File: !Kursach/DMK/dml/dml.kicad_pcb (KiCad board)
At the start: 2 copper layers, 64.7 x 68.8 mm, 26 parts, among them J1 Debug, J2 Conn_01x01_Male, J3 USB, SW1 SW_Push, SW2 SW_Push, U1 HEF4093B

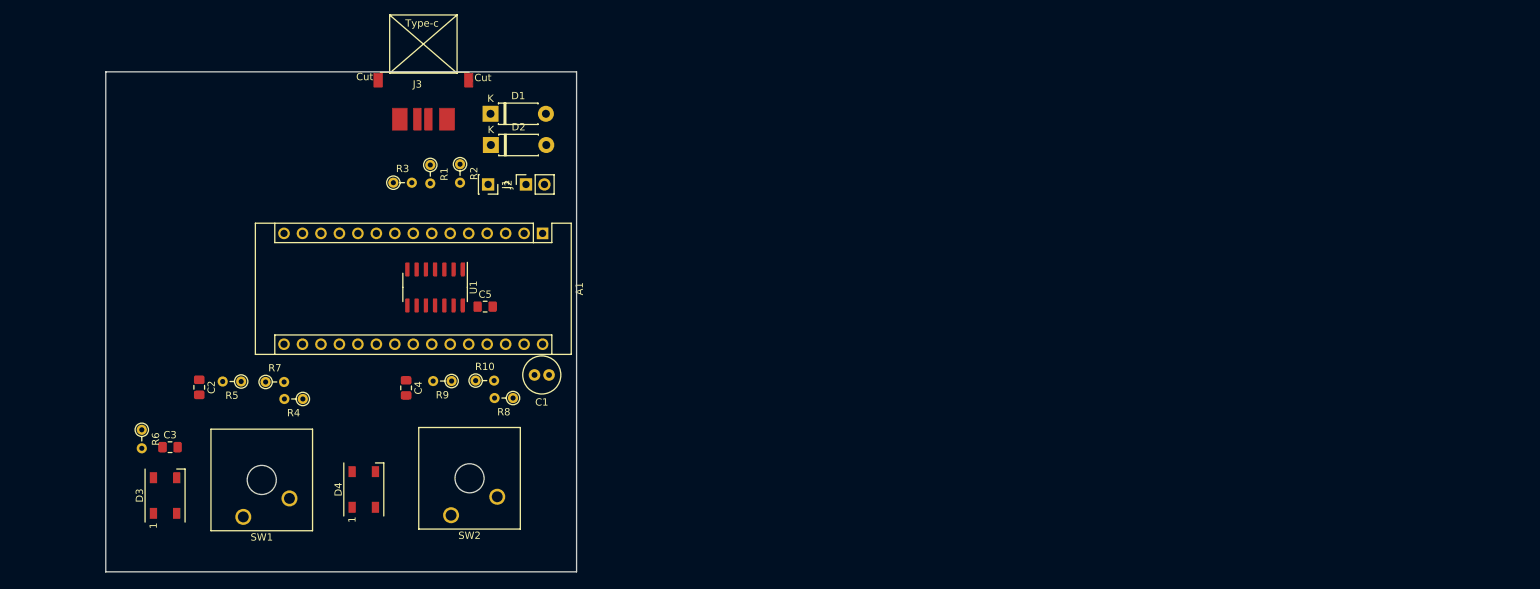
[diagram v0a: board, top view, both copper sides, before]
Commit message: s
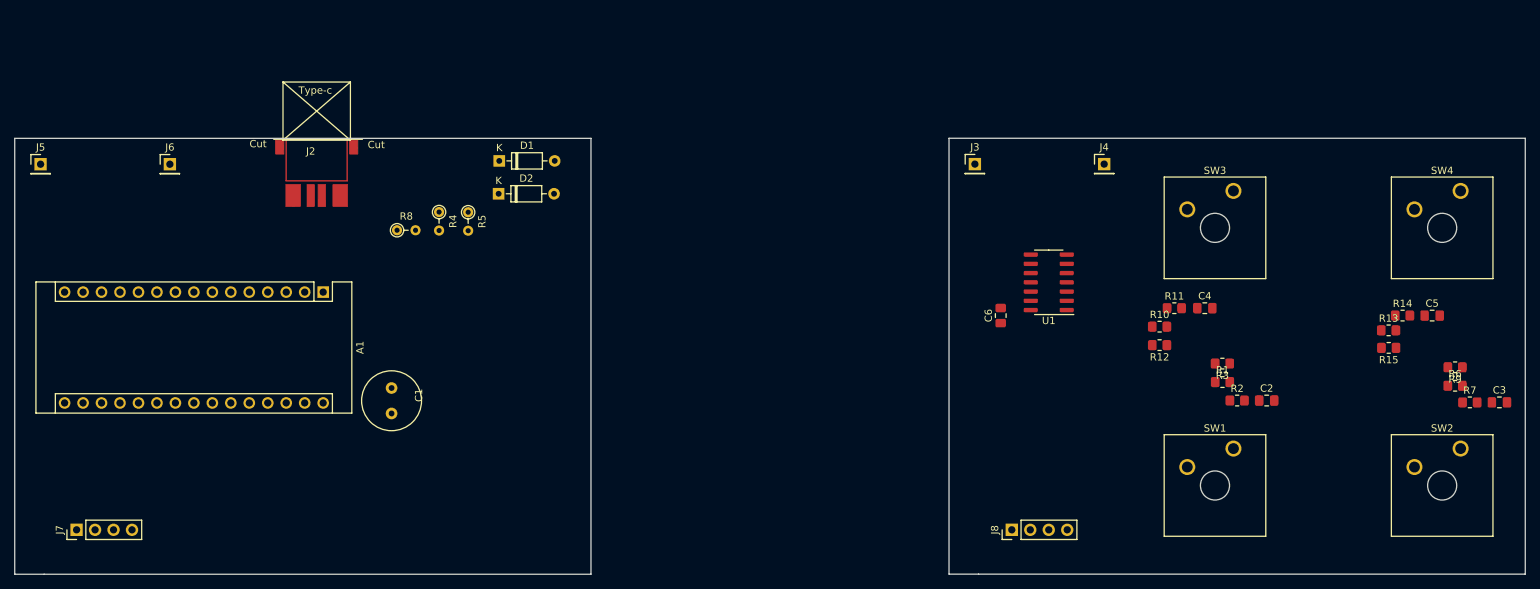
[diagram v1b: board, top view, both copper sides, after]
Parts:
- removed the C3 at (45.2, 62.5)
- removed D3, D4: WS2812B, LED_SMD:LED_WS2812B_PLCC4_5.0x5.0mm_P3.2mm
- removed J1: Debug, Connector_PinSocket_2.54mm:PinSocket_1x02_P2.54mm_Vertical
- removed the J2 at (89.0, 26.4)
- removed the R6 at (41.4, 60.1)
- added C4: 100nF???10nF, Capacitor_SMD:C_0805_2012Metric_Pad1.18x1.45mm_HandSolder, F.Cu at (187.5, 43.4)
- added C5: 100nF???10nF, Capacitor_SMD:C_0805_2012Metric_Pad1.18x1.45mm_HandSolder, F.Cu at (218.8, 44.4)
- added J3: Conn_01x01_Male, Connector_PinHeader_2.54mm:PinHeader_1x01_P2.54mm_Vertical, F.Cu at (155.9, 23.6)
- added J4: Conn_01x01_Male, Connector_PinHeader_2.54mm:PinHeader_1x01_P2.54mm_Vertical, F.Cu at (173.7, 23.6)
- added J5: Conn_01x01_Female, Connector_PinHeader_2.54mm:PinHeader_1x01_P2.54mm_Vertical, F.Cu at (27.4, 23.6)
- added J6: Conn_01x01_Female, Connector_PinHeader_2.54mm:PinHeader_1x01_P2.54mm_Vertical, F.Cu at (45.2, 23.6)
- added J7: Conn_01x04_Male, Connector_PinHeader_2.54mm:PinHeader_1x04_P2.54mm_Vertical, F.Cu at (32.4, 73.9)
- added J8: Conn_01x04_Female, Connector_PinHeader_2.54mm:PinHeader_1x04_P2.54mm_Vertical, F.Cu at (161.0, 73.9)
- added R10: ???20k, Resistor_SMD:R_0805_2012Metric_Pad1.20x1.40mm_HandSolder, F.Cu at (181.3, 46.0)
- added R11: ???100k, Resistor_SMD:R_0805_2012Metric_Pad1.20x1.40mm_HandSolder, F.Cu at (183.3, 43.4)
- added R12: 2.2k, Resistor_SMD:R_0805_2012Metric_Pad1.20x1.40mm_HandSolder, F.Cu at (181.3, 48.5)
- added R13: ???20k, Resistor_SMD:R_0805_2012Metric_Pad1.20x1.40mm_HandSolder, F.Cu at (212.8, 46.5)
- added R14: ???100k, Resistor_SMD:R_0805_2012Metric_Pad1.20x1.40mm_HandSolder, F.Cu at (214.7, 44.4)
- added R15: 2.2k, Resistor_SMD:R_0805_2012Metric_Pad1.20x1.40mm_HandSolder, F.Cu at (212.8, 48.9)
- added SW3: SW_Push, Button_Switch_Keyboard:SW_Cherry_MX_1.00u_Plate, F.Cu at (191.5, 27.3)
- added SW4: SW_Push, Button_Switch_Keyboard:SW_Cherry_MX_1.00u_Plate, F.Cu at (222.7, 27.3)
- C1: footprint Capacitor_THT:C_Radial_D5.0mm_H11.0mm_P2.00mm -> Capacitor_THT:C_Radial_D8.0mm_H7.0mm_P3.50mm
- D1, D2: footprint Diode_THT:D_DO-41_SOD81_P7.62mm_Horizontal -> Diode_THT:D_DO-35_SOD27_P7.62mm_Horizontal
- R1: renamed from R4; footprint Resistor_THT:R_Axial_DIN0204_L3.6mm_D1.6mm_P2.54mm_Vertical -> Resistor_SMD:R_0805_2012Metric_Pad1.20x1.40mm_HandSolder
- R2: renamed from R5; footprint Resistor_THT:R_Axial_DIN0204_L3.6mm_D1.6mm_P2.54mm_Vertical -> Resistor_SMD:R_0805_2012Metric_Pad1.20x1.40mm_HandSolder
- R3: renamed from R7; footprint Resistor_THT:R_Axial_DIN0204_L3.6mm_D1.6mm_P2.54mm_Vertical -> Resistor_SMD:R_0805_2012Metric_Pad1.20x1.40mm_HandSolder
- R6: renamed from R8; footprint Resistor_THT:R_Axial_DIN0204_L3.6mm_D1.6mm_P2.54mm_Vertical -> Resistor_SMD:R_0805_2012Metric_Pad1.20x1.40mm_HandSolder
- R7: renamed from R9; footprint Resistor_THT:R_Axial_DIN0204_L3.6mm_D1.6mm_P2.54mm_Vertical -> Resistor_SMD:R_0805_2012Metric_Pad1.20x1.40mm_HandSolder
- R9: renamed from R10; footprint Resistor_THT:R_Axial_DIN0204_L3.6mm_D1.6mm_P2.54mm_Vertical -> Resistor_SMD:R_0805_2012Metric_Pad1.20x1.40mm_HandSolder
- moved C3 150.4 mm to (228.1, 56.4), turned to 0 degrees
- moved C2 146.8 mm to (196.0, 56.1), turned to 0 degrees
- moved R7 140.1 mm to (224.0, 56.4), turned to 0 degrees
- moved SW2 139.1 mm to (222.7, 62.7), turned to 0 degrees
- moved R2 137.0 mm to (192.0, 56.1), turned to 0 degrees
- moved SW1 136.5 mm to (191.5, 62.7), turned to 0 degrees
- moved R9 134.7 mm to (222.0, 51.5), turned to 180 degrees
- moved R3 131.6 mm to (190.0, 51.0), turned to 180 degrees
- moved R6 129.6 mm to (222.0, 54.1), turned to 0 degrees
- moved R1 126.5 mm to (190.0, 53.6), turned to 0 degrees
- moved U1 84.4 mm to (166.1, 39.9), turned to 180 degrees
- moved C6 70.9 mm to (159.5, 44.4), turned to 90 degrees
- moved A1 31.2 mm to (66.3, 41.2)
- moved C1 21.7 mm to (75.7, 54.4), turned to 270 degrees
- moved J2 17.3 mm to (64.7, 21.0)
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- renumbered C4 to C3, C5 to C6, J3 to J2, R1 to R4, R2 to R5, R3 to R8
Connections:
- A1 pad 1: Net-(A1-Pad1) -> (no net)
- A1 pad 10: (no net) -> /Butt4
- A1 pad 11: /Led -> /Butt3
- A1 pad 12: (no net) -> /Butt2
- A1 pad 13: (no net) -> /Butt1
- A1 pad 2: Net-(A1-Pad2) -> (no net)
- A1 pad 6: /Butt1 -> (no net)
- A1 pad 9: /Butt2 -> (no net)
- U1 pad 10: (no net) -> /Butt3
- U1 pad 11: (no net) -> /Butt4
- U1 pad 12: (no net) -> Net-(R15-Pad2)
- U1 pad 13: (no net) -> Net-(R15-Pad2)
- U1 pad 8: (no net) -> Net-(R12-Pad2)
- U1 pad 9: (no net) -> Net-(R12-Pad2)
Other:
- board size 64.7 x 68.8 mm -> 207.7 x 60 mm
